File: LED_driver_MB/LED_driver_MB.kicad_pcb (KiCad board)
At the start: 2 copper layers, 77 x 94.5 mm, 75 parts, among them J1 Conn_01x03_Socket, J2 Conn_01x03_Socket, J3 Conn_01x03_Socket, J4 Conn_01x02_Socket, J5 Conn_01x03_Socket, J6 Conn_01x06, Q1 IRLZ44NPBF, Q10 BC847, Q11 IRLZ44NPBF, Q12 BC847, Q2 BC847, Q3 IRLZ44NPBF, Q4 BC847, Q5 IRLZ44NPBF, Q6 BC847, Q7 IRLZ44NPBF, Q8 BC847, Q9 IRLZ44NPBF, SW1 SW_SPDT, SW2 SW_SPST, SW3 SW_SPST, SW4 SW_SPST, U1 ESP32-C3_SUPERMINI_TH, U6 TPS563201

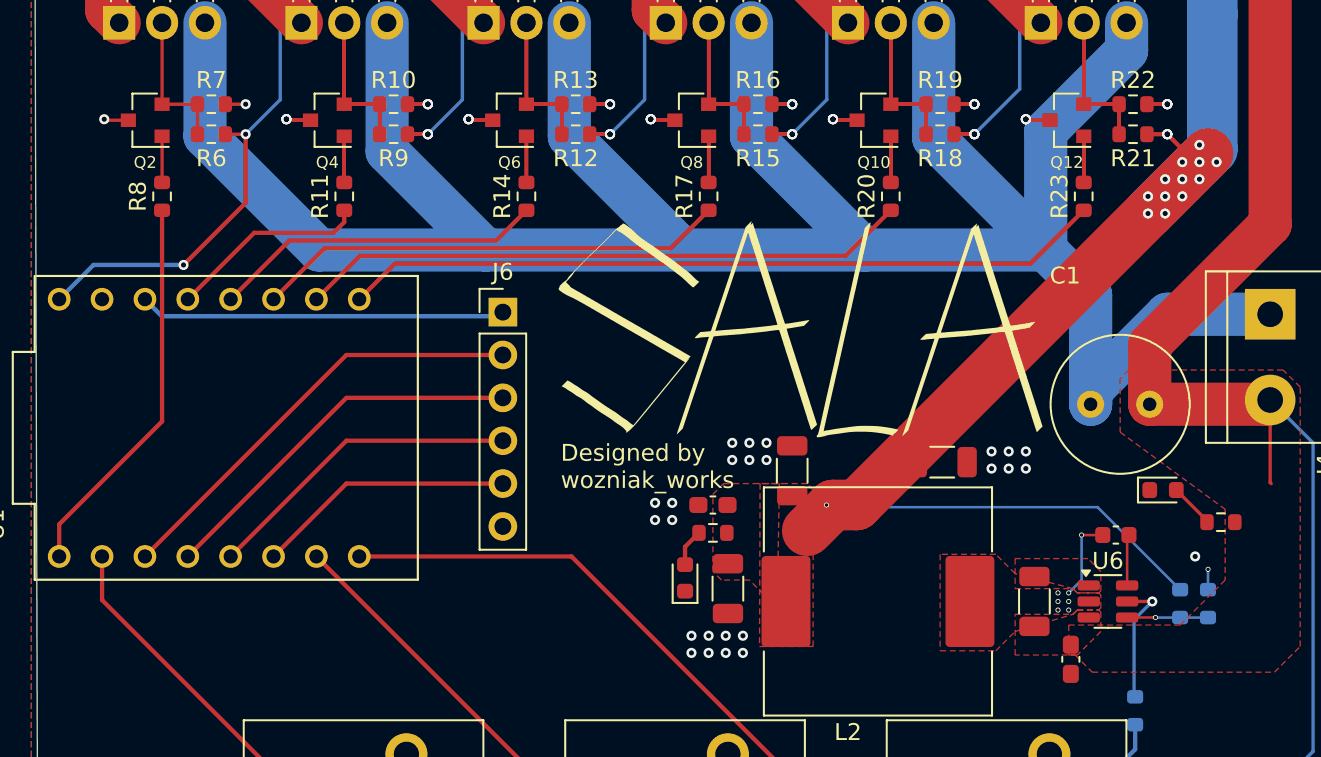
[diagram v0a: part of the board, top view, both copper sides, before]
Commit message: Via size unified
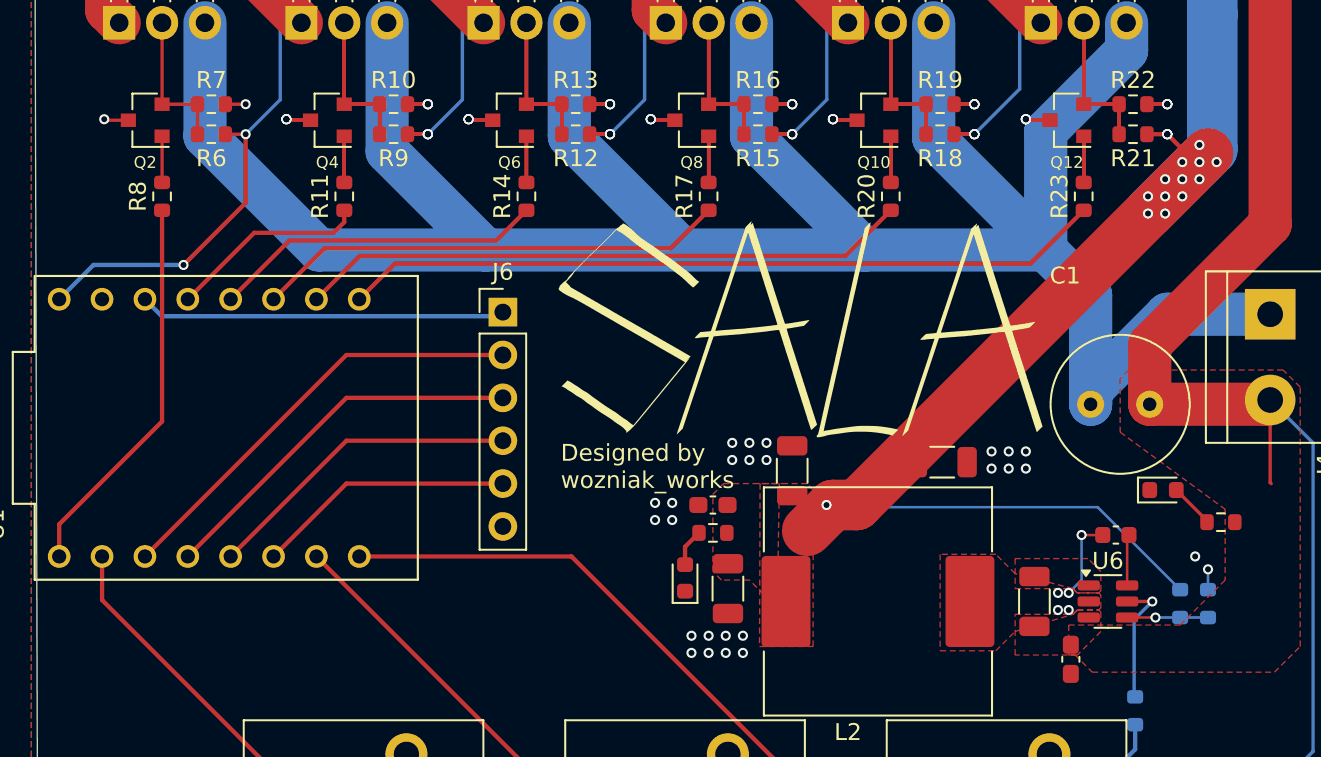
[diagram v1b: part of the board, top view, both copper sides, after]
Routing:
- net Net-(U6-SW): vias 7 -> 5
